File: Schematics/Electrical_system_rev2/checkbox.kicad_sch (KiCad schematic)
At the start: 28 parts, among them K6 Relay_SPST-NO, U10 TSAL, U8 BSPD, U9 Relay board

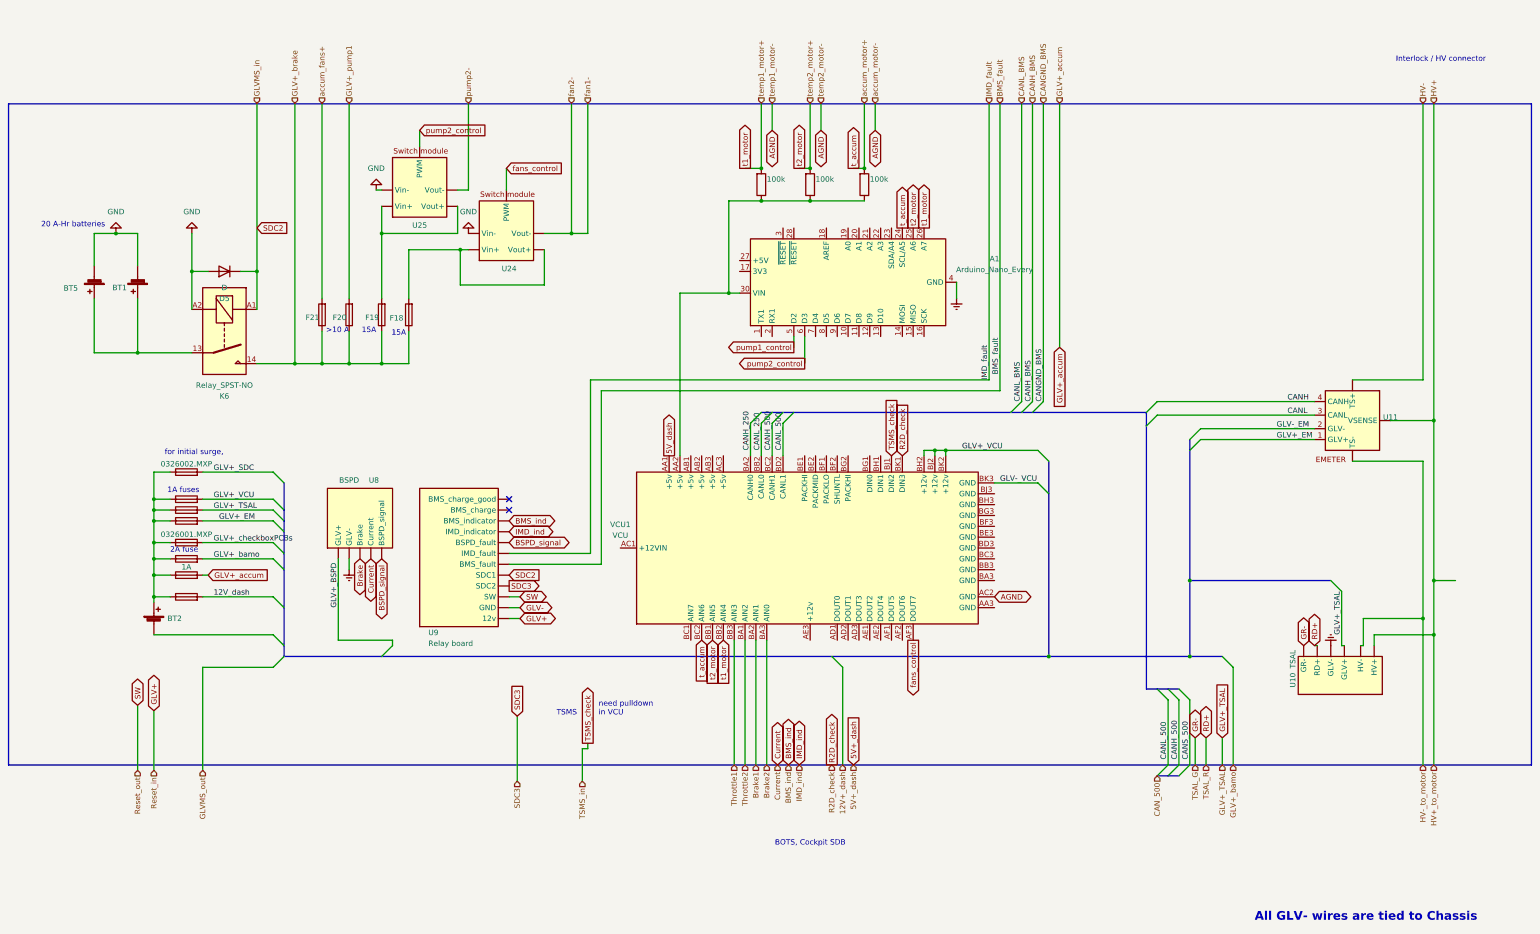
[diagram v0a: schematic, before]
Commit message: updating of electrical system
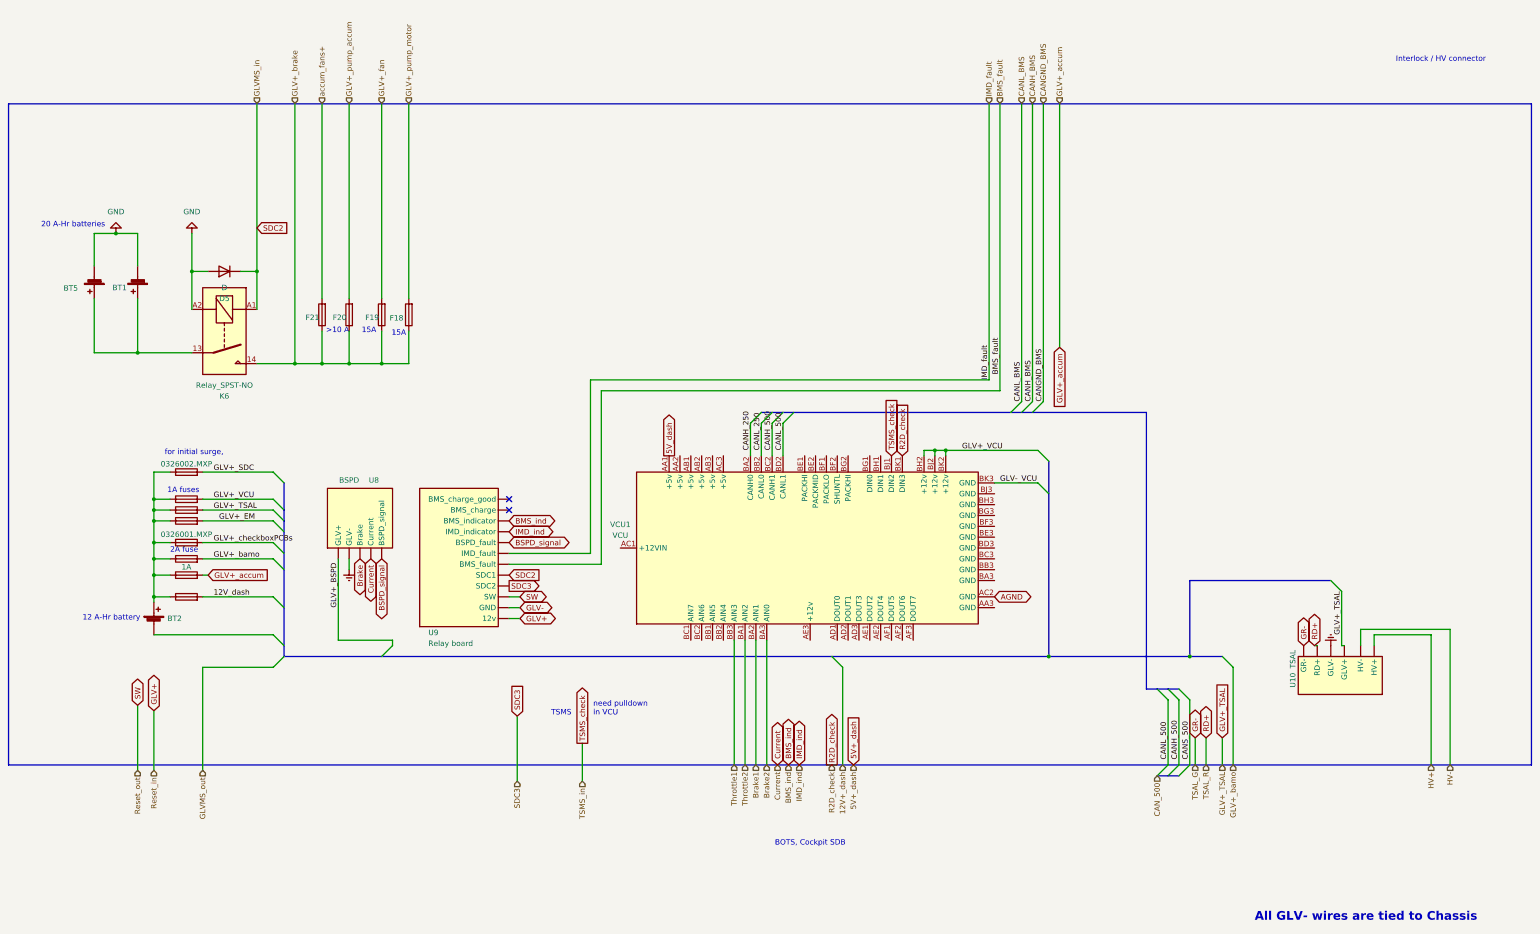
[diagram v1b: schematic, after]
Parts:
- removed A1: Arduino_Nano_Every, Module:Arduino_Nano, symbol MCU_Module:Arduino_Nano_Every
- removed R4, R5, R6: 100k, symbol Device:R
- removed U11: ~, symbol FSAE:Emeter
- removed U24, U25: ~, symbol FSAE:switch_moduel
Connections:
- net HV-_to_motor is gone; now on net RD+: U10. (RD+)
- net t1_motor is gone; now on net CANL_250: VCU1.BB2 (CANL0)
- net t_accum is gone; now on net CANH_500: VCU1.BC2 (CANH1)
- net HV-: now also U10. (RD+)
- net GLV+_pump_motor: now reaches F18.2
- net GLV+_fan: now reaches F19.2
- net GLV+_pump1 renamed GLV+_pump_accum
- net fans_control: no longer names the net of VCU1.AF3 (DOUT7)
- net t2_motor: no longer names the net of VCU1.BB1 (AIN5)
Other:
- note added: "12 A-Hr battery"
